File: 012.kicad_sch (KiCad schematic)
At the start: 1 part, among them U1 AM6232ASCGHAALWR

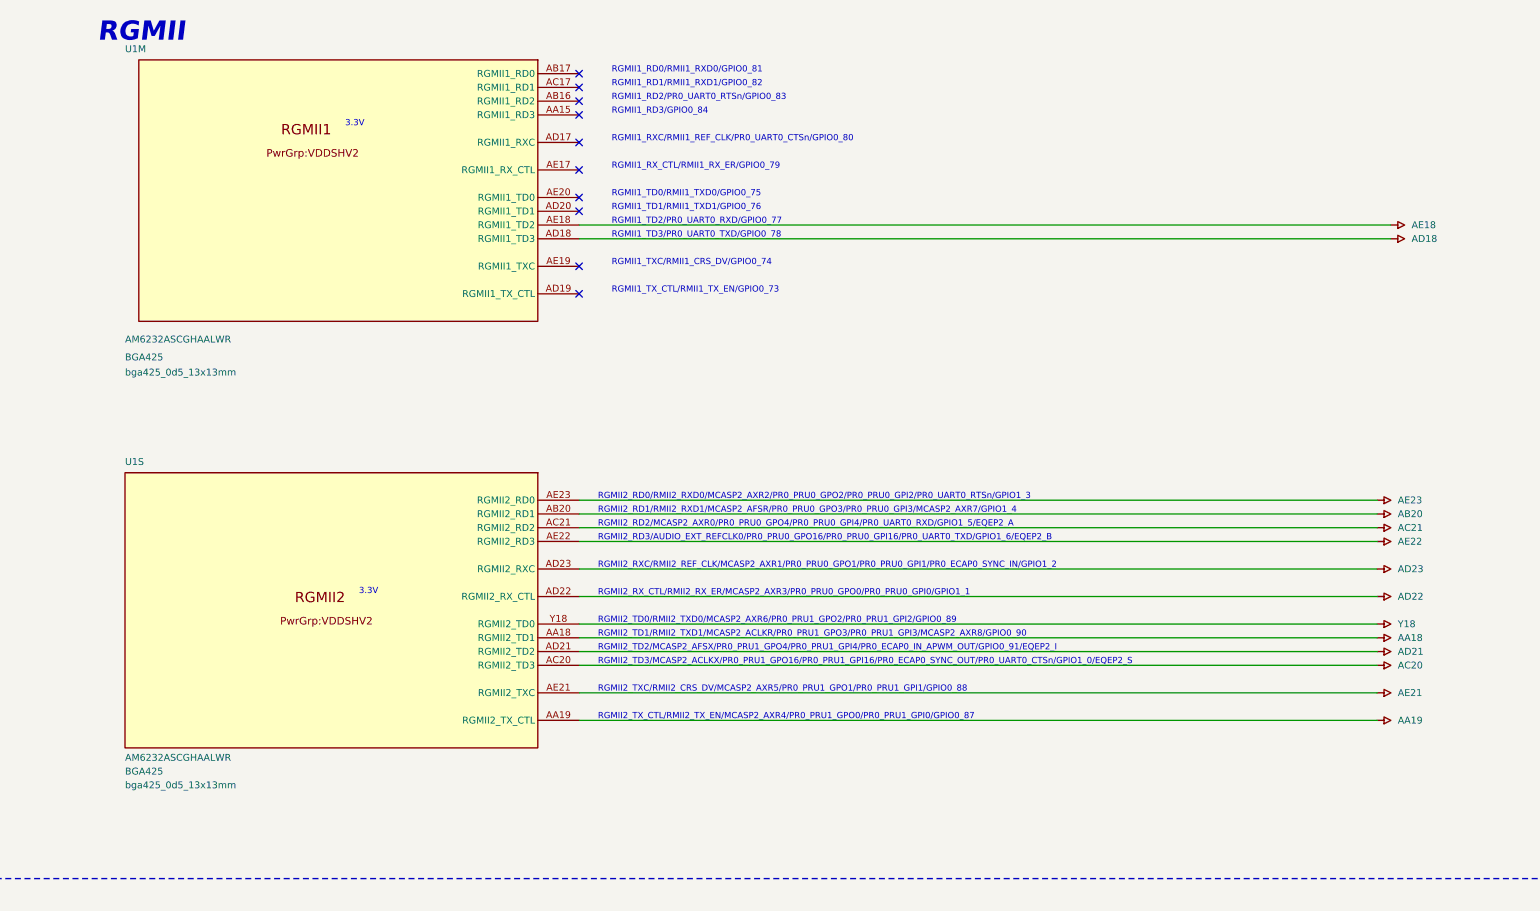
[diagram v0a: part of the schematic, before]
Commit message: Another round of cleansing fire
Signed-off-by: Michael Welling <mwelling79@gmail.com>
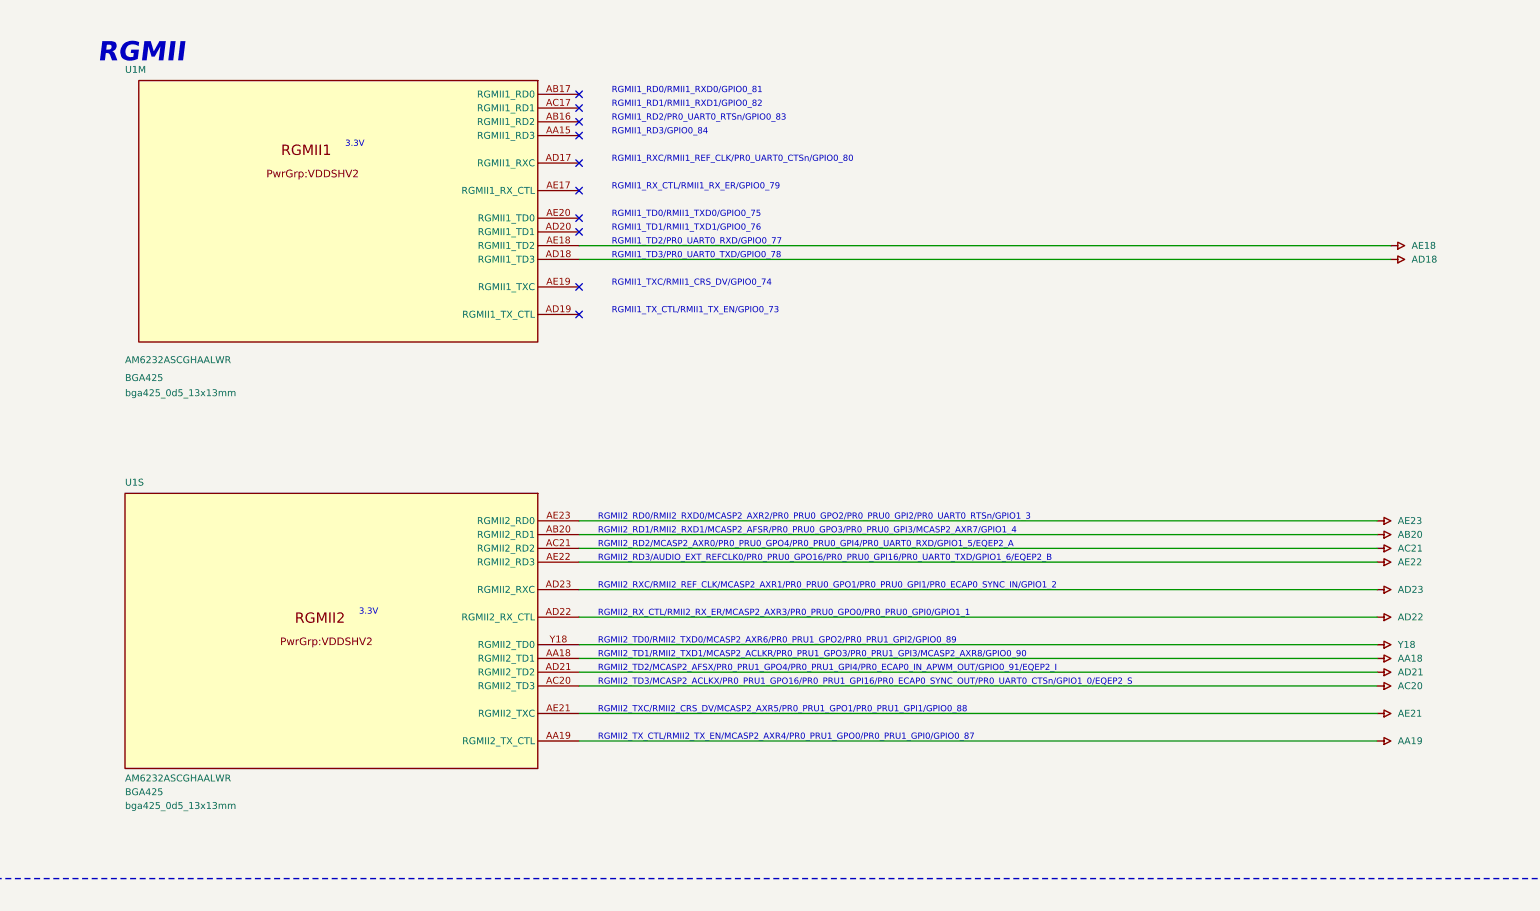
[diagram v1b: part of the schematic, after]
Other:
- moved on the sheet: U1M, U1S
